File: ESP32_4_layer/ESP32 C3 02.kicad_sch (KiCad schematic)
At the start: 15 parts, among them J3 GSD090012SEU_SDcard_Connector, U2 ESP32-C3-WROOM-02, U3 CP2102N-Axx-xQFN20, U4 USBLC6-2SC6, U5 W25Q32JVSS

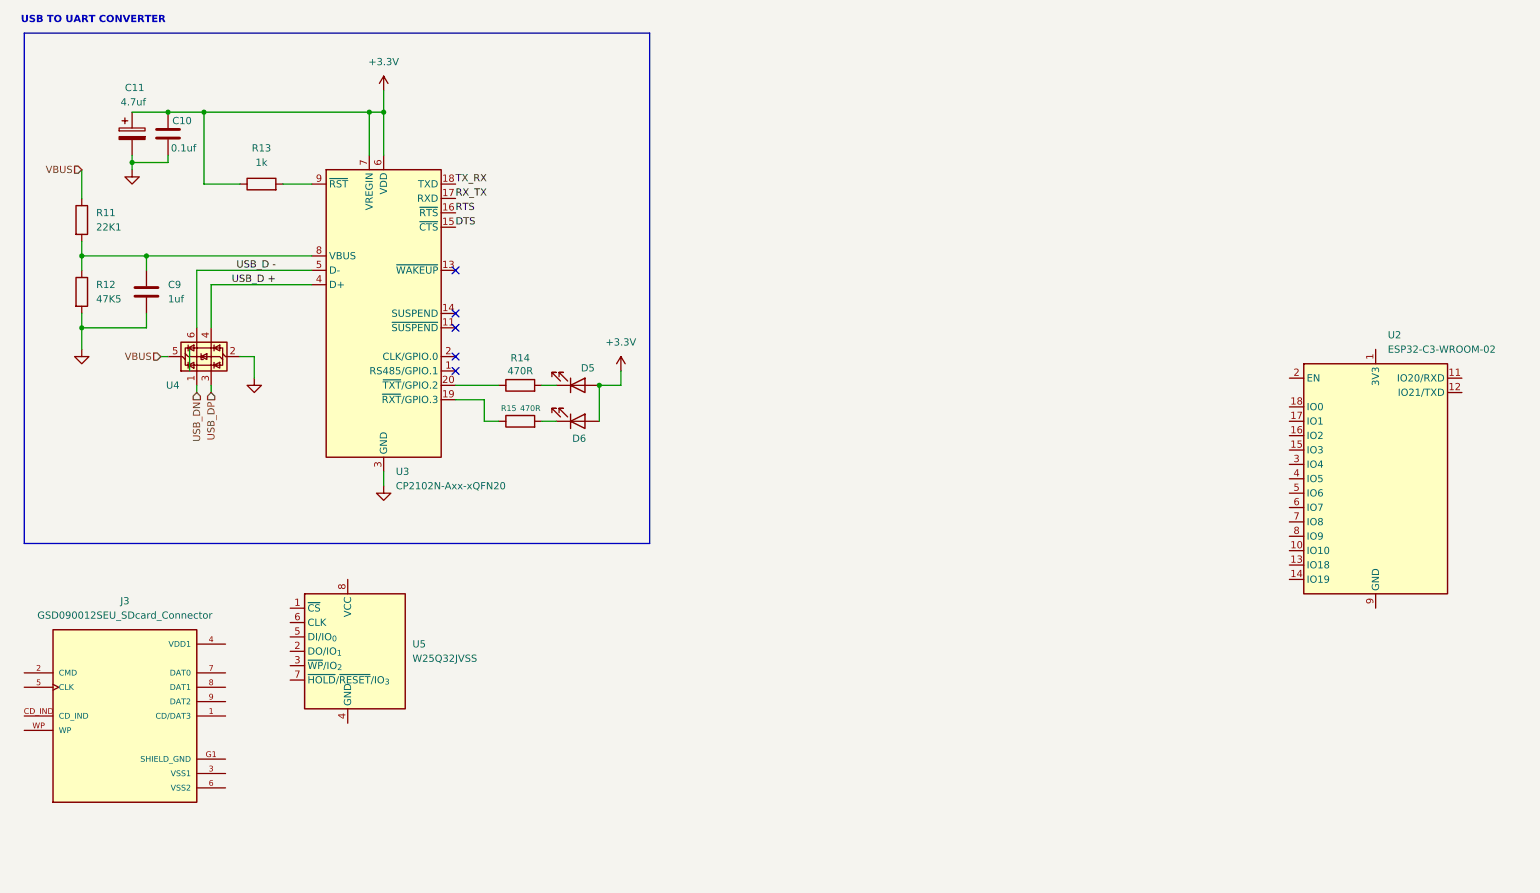
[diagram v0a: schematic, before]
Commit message: MCU and SD CARD schematic completed
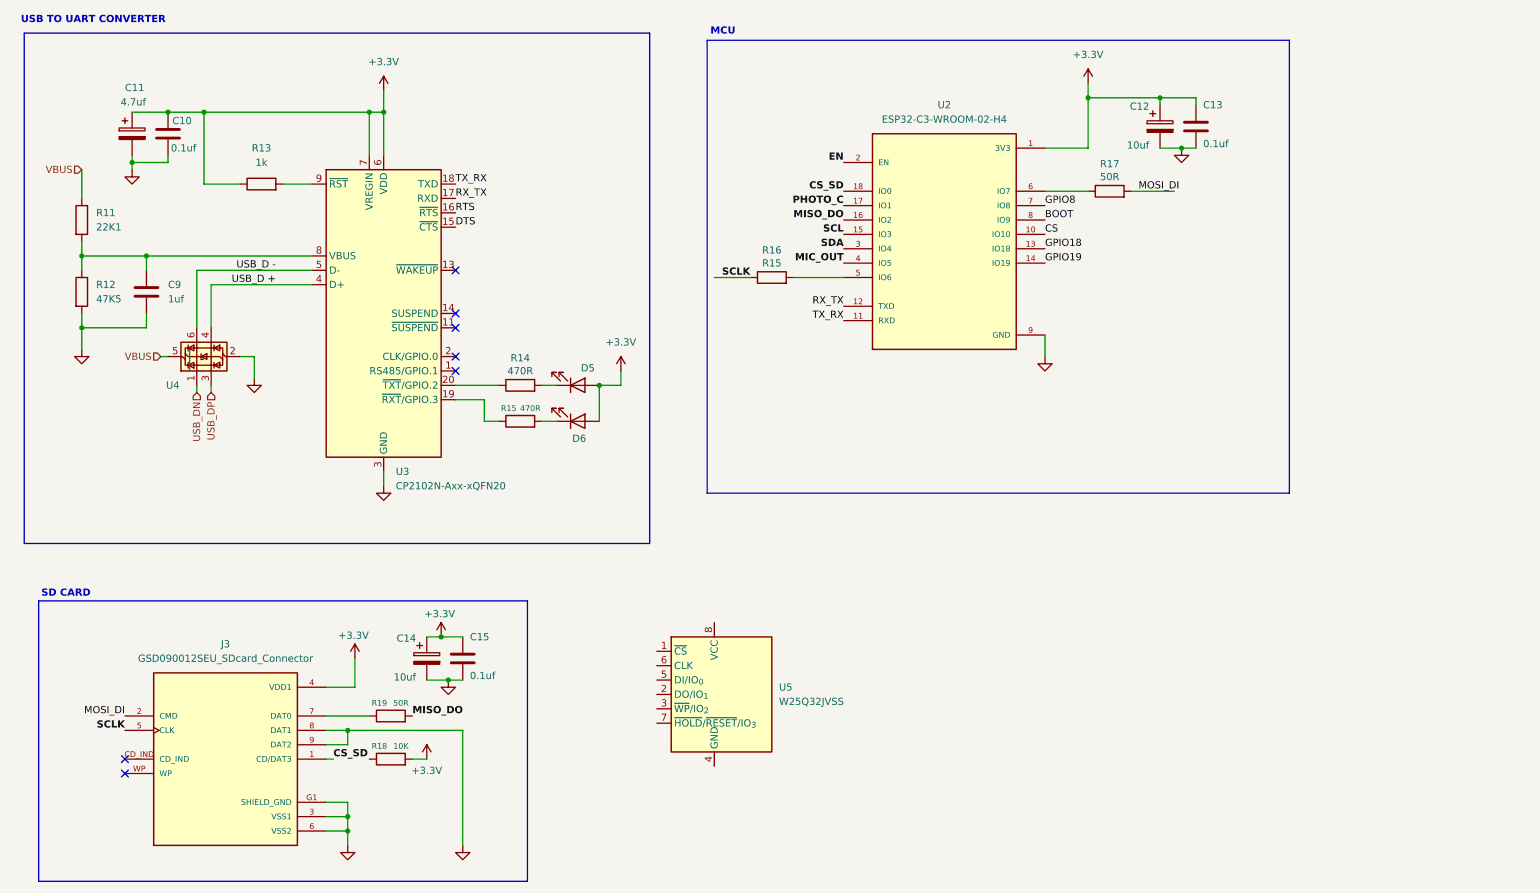
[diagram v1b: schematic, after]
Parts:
- removed U2: ESP32-C3-WROOM-02, RF_Module:ESP32-C3-WROOM-02, symbol RF_Module:ESP32-C3-WROOM-02
- added C12, C14: 10uf, symbol Device:C_Polarized
- added C13, C15: 0.1uf, symbol Device:C
- added R16: R15, symbol Device:R
- added R17, R19: 50R, symbol Device:R
- added R18: 10K, symbol Device:R
- added U2: ESP32-C3-WROOM-02-H4, ESP32-C3-WROOM-02-H4:MODULE_ESP32-C3-WROOM-02-H4, symbol Own_Library:ESP32-C3-WROOM-02-H4
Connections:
- net SHIELD_GND is gone; now on net GND: J3.G1 (SHIELD_GND), J3.G2 (SHIELD_GND), J3.G3 (SHIELD_GND), J3.G4 (SHIELD_GND)
- net +3.3V: now also J3.4 (VDD1), C12.1, C13.1, C14.1, C15.1, R18.2, U2.1 (3V3)
- net GND: now also J3.3 (VSS1), J3.6 (VSS2), J3.8 (DAT1), J3.9 (DAT2), C12.2, C13.2, C14.2, C15.2, U2.19 (GND), U2.20 (GND), U2.21 (GND), U2.22 (GND), U2.23 (GND), U2.24 (GND), U2.25 (GND), U2.26 (GND), U2.27 (GND), U2.28 (GND), U2.29 (GND), U2.30 (GND), U2.31 (GND), U2.32 (GND), U2.33 (GND), U2.34 (GND), U2.35 (GND), U2.36 (GND), U2.37 (GND), U2.38 (GND), U2.39 (GND), U2.9 (GND)
- net RX_TX: now also U2.12 (TXD)
- net TX_RX: now also U2.11 (RXD)
- net CS_SD: now reaches J3.1 (CD/DAT3)
- net CS_SD: now also U2.18 (IO0)
- net MOSI_DI: now reaches J3.2 (CMD)
- net MOSI_DI: now also R17.2
- net SCLK: now reaches J3.5 (CLK)
- net SCLK: now also R16.1
- net at J3.7 (DAT0): now also R19.1
- new net: R17.1, U2.6 (IO7)
- new net: R16.2, U2.5 (IO6)
- new net BOOT: U2.8 (IO9)
- new net CS: U2.10 (IO10)
- new net EN: U2.2 (EN)
- new net GPIO18: U2.13 (IO18)
- new net GPIO19: U2.14 (IO19)
- new net GPIO8: U2.7 (IO8)
- new net MIC_OUT: U2.4 (IO5)
- new net MISO_DO: R19.2, U2.16 (IO2)
- new net PHOTO_C: U2.17 (IO1)
- new net SCL: U2.15 (IO3)
- new net SDA: U2.3 (IO4)
- no-connect marks 5 -> 7
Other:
- note added: "MCU"
- note added: "SD CARD"
- moved on the sheet: J3, U5

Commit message: FLASH AND TEST POINTS
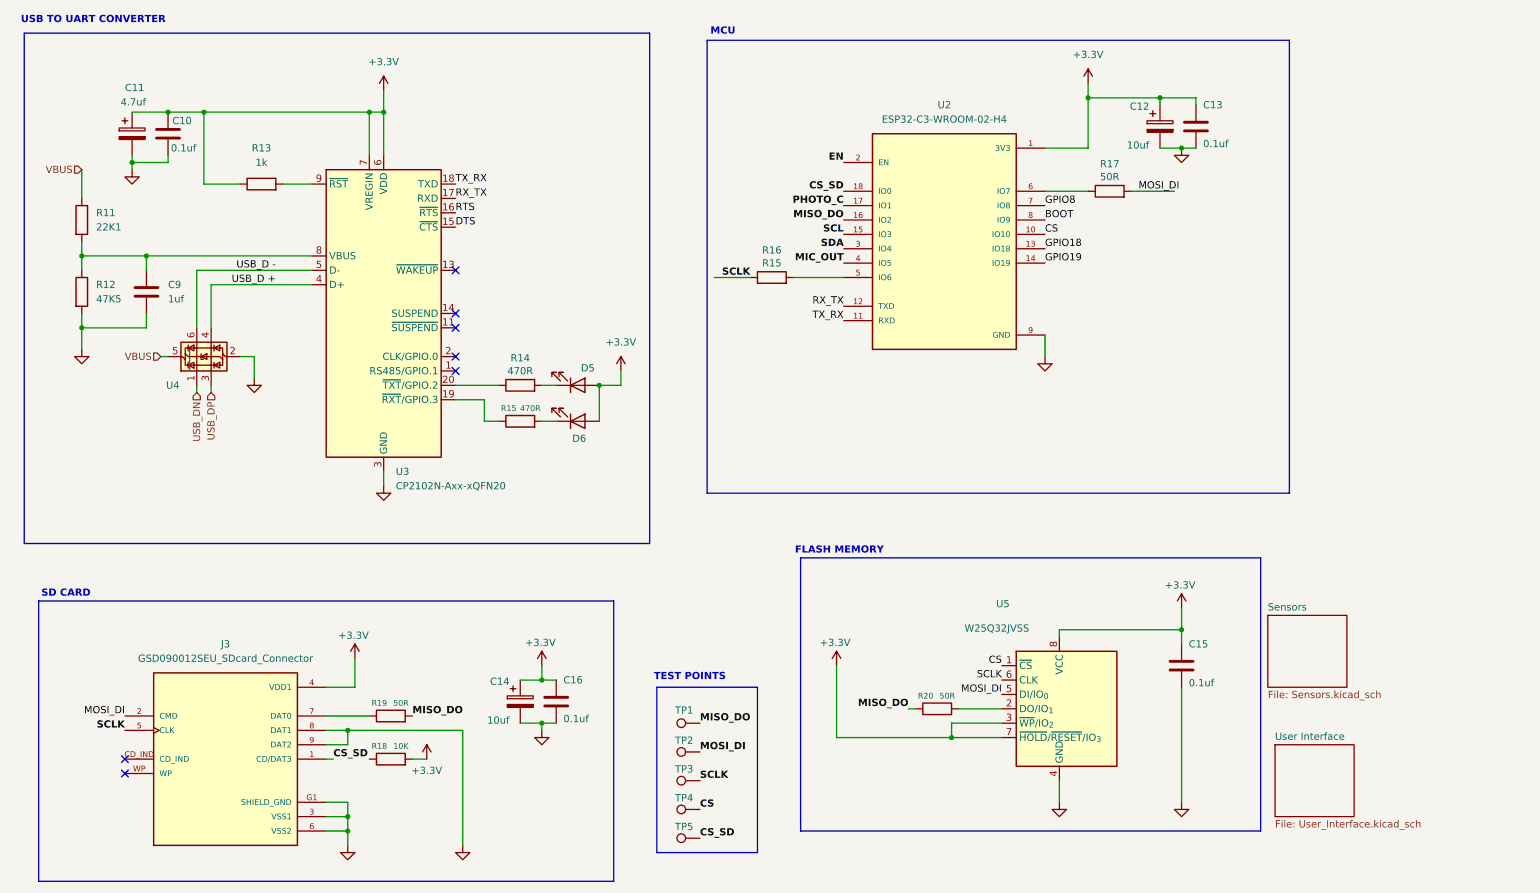
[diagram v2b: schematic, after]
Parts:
- added C16: 0.1uf, symbol Device:C
- added R20: 50R, symbol Device:R
- added TP1, TP2, TP3, TP4, TP5: TestPoint, symbol Connector:TestPoint
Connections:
- net +3.3V: now also U5.3 (~{WP}/IO_{2}), U5.7 (~{HOLD}/~{RESET}/IO_{3}), U5.8 (VCC), C16.1
- net CS: now also U5.1 (~{CS}), TP4.1
- net CS_SD: now also TP5.1
- net GND: now also U5.4 (GND), C16.2
- net MISO_DO: now also R20.1, TP1.1
- net MOSI_DI: now also U5.5 (DI/IO_{0}), TP2.1
- net SCLK: now also U5.6 (CLK), TP3.1
- net at U5.2 (DO/IO_{1}): now also R20.2
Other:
- added sheet Sensors (Sensors.kicad_sch)
- added sheet User Interface (User_Interface.kicad_sch)
- note added: "FLASH MEMORY"
- note added: "TEST POINTS"
- title: (none) -> ESP32 C3, USB to UART, SD CARD and FLASH
- moved on the sheet: C15, U5

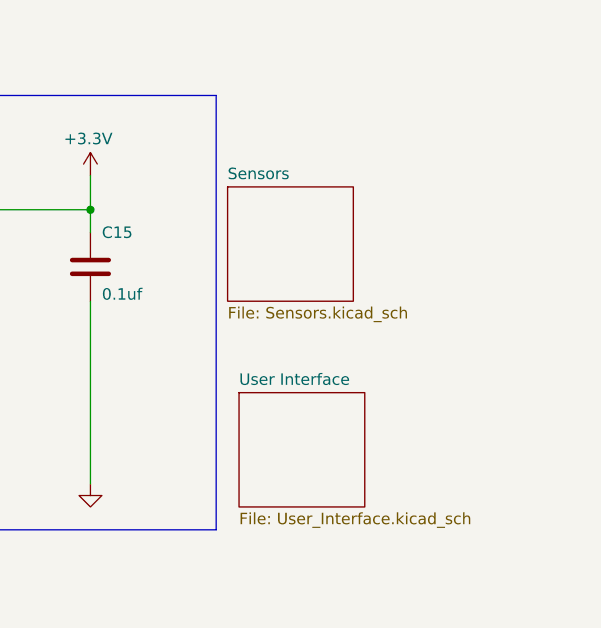
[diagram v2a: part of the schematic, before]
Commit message: SENSORS COMPLETED
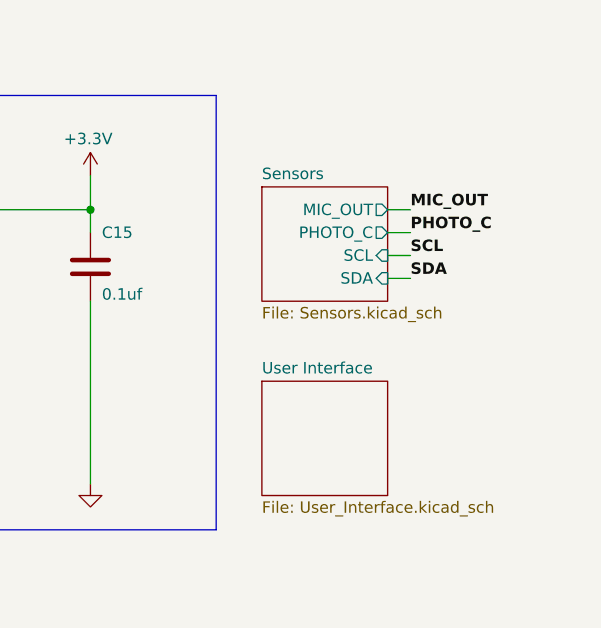
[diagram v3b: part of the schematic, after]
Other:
- sheet Sensors ports: added MIC_OUT, PHOTO_C, SCL, SDA; removed none
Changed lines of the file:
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@@
 	(wire
 		(pts
+			(xy 262.89 125.73) (xy 260.35 125.73)
+		)
+		(stroke
+			(width 0)
+			(type default)
+		)
+	)
+	(wire
+		(pts
 			(xy 205.74 156.21) (xy 205.74 152.4)
 		)
@@
 	(wire
 		(pts
+			(xy 262.89 133.35) (xy 260.35 133.35)
+		)
+		(stroke
+			(width 0)
+			(type default)
+		)
+	)
+	(wire
+		(pts
 			(xy 203.2 48.26) (xy 210.82 48.26)
 		)
@@
 	(wire
 		(pts
+			(xy 262.89 128.27) (xy 260.35 128.27)
+		)
+		(stroke
+			(width 0)
+			(type default)
+		)
+	)
+	(wire
+		(pts
 			(xy 48.26 41.91) (xy 48.26 43.18)
 		)
@@
 	(wire
 		(pts
+			(xy 262.89 130.81) (xy 260.35 130.81)
+		)
+		(stroke
+			(width 0)
+			(type default)
+		)
+	)
+	(wire
+		(pts
 			(xy 48.26 34.29) (xy 54.61 34.29)
 		)
@@
 		)
 	)
+	(label "SDA"
+		(at 262.89 133.35 0)
+		(effects
+			(font
+				(size 1.27 1.27)
+				(thickness 0.254)
+				(bold yes)
+			)
+			(justify left bottom)
+		)
+	)
+	(label "MIC_OUT"
+		(at 262.89 125.73 0)
+		(effects
+			(font
+				(size 1.27 1.27)
+				(thickness 0.254)
+				(bold yes)
+			)
+			(justify left bottom)
+		)
+	)
 	(label "GPIO18"
 		(at 203.2 58.42 0)
@@
 		)
 	)
+	(label "SCL"
+		(at 262.89 130.81 0)
+		(effects
+			(font
+				(size 1.27 1.27)
+				(thickness 0.254)
+				(bold yes)
+			)
+			(justify left bottom)
+		)
+	)
 	(label "MOSI_DI"
 		(at 219.71 48.26 0)
@@
 		)
 	)
+	(label "PHOTO_C"
+		(at 262.89 128.27 0)
+		(effects
+			(font
+				(size 1.27 1.27)
+				(thickness 0.254)
+				(bold yes)
+			)
+			(justify left bottom)
+		)
+	)
 	(label "MISO_DO"
 		(at 167.64 53.34 180)
@@
 	)
 	(sheet
-		(at 243.84 146.05)
+		(at 246.38 144.78)
 		(size 13.97 12.7)
 		(exclude_from_sim no)
@@
 		)
 		(property "Sheetname" "User Interface"
-			(at 243.84 145.3384 0)
+			(at 246.38 144.0684 0)
 			(effects
 				(font
@@
 		)
 		(property "Sheetfile" "User_Interface.kicad_sch"
-			(at 243.84 159.3346 0)
+			(at 246.38 158.0646 0)
 			(effects
 				(font
@@
 	)
 	(sheet
-		(at 242.57 123.19)
+		(at 246.38 123.19)
 		(size 13.97 12.7)
 		(exclude_from_sim no)
@@
 		)
 		(fill
-			(color 37 17 255 1.0000)
+			(color 39 252 255 1.0000)
 		)
 		(property "Sheetname" "Sensors"
-			(at 242.57 122.4784 0)
+			(at 246.38 122.4784 0)
 			(effects
 				(font
@@
 		)
 		(property "Sheetfile" "Sensors.kicad_sch"
-			(at 242.57 136.4746 0)
+			(at 246.38 136.4746 0)
 			(effects
 				(font
@@
 			)
 		)
+		(pin "MIC_OUT" output
+			(at 260.35 125.73 0)
+			(effects
+				(font
+					(size 1.27 1.27)
+				)
+				(justify right)
+			)
+		)
+		(pin "PHOTO_C" output
+			(at 260.35 128.27 0)
+			(effects
+				(font
+					(size 1.27 1.27)
+				)
+				(justify right)
+			)
+		)
+		(pin "SCL" input
+			(at 260.35 130.81 0)
+			(effects
+				(font
+					(size 1.27 1.27)
+				)
+				(justify right)
+			)
+		)
+		(pin "SDA" input
+			(at 260.35 133.35 0)
+			(effects
+				(font
+					(size 1.27 1.27)
+				)
+				(justify right)
+			)
+		)
